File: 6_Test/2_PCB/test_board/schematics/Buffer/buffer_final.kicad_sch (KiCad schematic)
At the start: 15 parts, among them U1 SN74ALVCH162827DLR

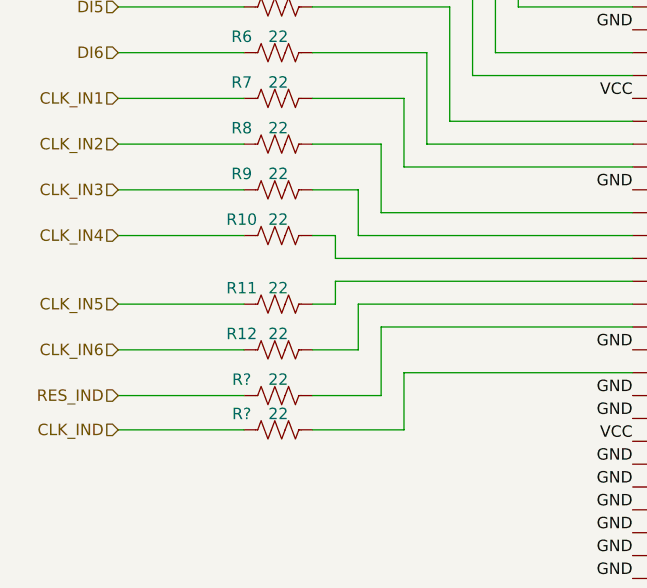
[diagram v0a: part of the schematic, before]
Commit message: Corrections to schematic 11_20_24
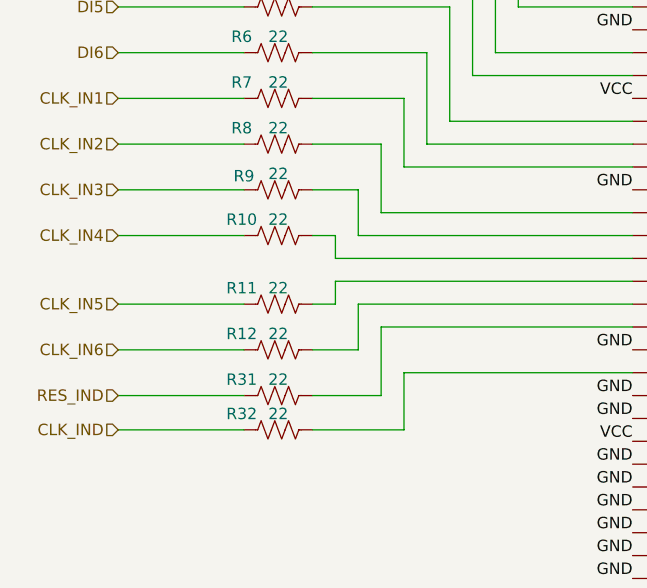
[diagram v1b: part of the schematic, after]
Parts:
- gave numbers to parts that had none: 2
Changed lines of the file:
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@@
 				)
 			)
-			(project "board_main_sim"
-				(path "/9c0580c5-7bd5-4e54-bf4c-826aa4ac3630/49c5ff04-0c5f-41d0-9aa9-a7998c02a6ab"
-					(reference "R10")
+			(project "board_main"
+				(path "/9c0580c5-7bd5-4e54-bf4c-826aa4ac3630/49c5ff04-0c5f-41d0-9aa9-a7998c02a6ab"
+					(reference "R20")
 					(unit 1)
 				)
@@
 				)
 			)
-			(project "board_main_sim"
-				(path "/9c0580c5-7bd5-4e54-bf4c-826aa4ac3630/49c5ff04-0c5f-41d0-9aa9-a7998c02a6ab"
-					(reference "R19")
+			(project "board_main"
+				(path "/9c0580c5-7bd5-4e54-bf4c-826aa4ac3630/49c5ff04-0c5f-41d0-9aa9-a7998c02a6ab"
+					(reference "R29")
 					(unit 1)
 				)
@@
 				)
 			)
-			(project "board_main_sim"
-				(path "/9c0580c5-7bd5-4e54-bf4c-826aa4ac3630/49c5ff04-0c5f-41d0-9aa9-a7998c02a6ab"
-					(reference "R9")
+			(project "board_main"
+				(path "/9c0580c5-7bd5-4e54-bf4c-826aa4ac3630/49c5ff04-0c5f-41d0-9aa9-a7998c02a6ab"
+					(reference "R19")
 					(unit 1)
 				)
@@
 				)
 			)
-			(project "board_main_sim"
-				(path "/9c0580c5-7bd5-4e54-bf4c-826aa4ac3630/49c5ff04-0c5f-41d0-9aa9-a7998c02a6ab"
-					(reference "R12")
+			(project "board_main"
+				(path "/9c0580c5-7bd5-4e54-bf4c-826aa4ac3630/49c5ff04-0c5f-41d0-9aa9-a7998c02a6ab"
+					(reference "R22")
 					(unit 1)
 				)
@@
 				)
 			)
-			(project "board_main_sim"
-				(path "/9c0580c5-7bd5-4e54-bf4c-826aa4ac3630/49c5ff04-0c5f-41d0-9aa9-a7998c02a6ab"
-					(reference "R14")
+			(project "board_main"
+				(path "/9c0580c5-7bd5-4e54-bf4c-826aa4ac3630/49c5ff04-0c5f-41d0-9aa9-a7998c02a6ab"
+					(reference "R24")
 					(unit 1)
 				)
@@
 				)
 			)
-			(project "board_main_sim"
-				(path "/9c0580c5-7bd5-4e54-bf4c-826aa4ac3630/49c5ff04-0c5f-41d0-9aa9-a7998c02a6ab"
-					(reference "R20")
+			(project "board_main"
+				(path "/9c0580c5-7bd5-4e54-bf4c-826aa4ac3630/49c5ff04-0c5f-41d0-9aa9-a7998c02a6ab"
+					(reference "R30")
 					(unit 1)
 				)
@@
 				)
 			)
-			(project "board_main_sim"
-				(path "/9c0580c5-7bd5-4e54-bf4c-826aa4ac3630/49c5ff04-0c5f-41d0-9aa9-a7998c02a6ab"
-					(reference "R13")
+			(project "board_main"
+				(path "/9c0580c5-7bd5-4e54-bf4c-826aa4ac3630/49c5ff04-0c5f-41d0-9aa9-a7998c02a6ab"
+					(reference "R23")
 					(unit 1)
 				)
@@
 		(dnp no)
 		(property "Reference" "R9"
-			(at 84.836 82.042 90)
+			(at 85.09 82.296 90)
 			(effects
 				(font
@@
 				)
 			)
-			(project "board_main_sim"
-				(path "/9c0580c5-7bd5-4e54-bf4c-826aa4ac3630/49c5ff04-0c5f-41d0-9aa9-a7998c02a6ab"
-					(reference "R17")
+			(project "board_main"
+				(path "/9c0580c5-7bd5-4e54-bf4c-826aa4ac3630/49c5ff04-0c5f-41d0-9aa9-a7998c02a6ab"
+					(reference "R27")
 					(unit 1)
 				)
@@
 				)
 			)
-			(project "board_main_sim"
-				(path "/9c0580c5-7bd5-4e54-bf4c-826aa4ac3630/49c5ff04-0c5f-41d0-9aa9-a7998c02a6ab"
-					(reference "R18")
+			(project "board_main"
+				(path "/9c0580c5-7bd5-4e54-bf4c-826aa4ac3630/49c5ff04-0c5f-41d0-9aa9-a7998c02a6ab"
+					(reference "R28")
 					(unit 1)
 				)
@@
 				)
 			)
-			(project "board_main_sim"
-				(path "/9c0580c5-7bd5-4e54-bf4c-826aa4ac3630/49c5ff04-0c5f-41d0-9aa9-a7998c02a6ab"
-					(reference "R15")
+			(project "board_main"
+				(path "/9c0580c5-7bd5-4e54-bf4c-826aa4ac3630/49c5ff04-0c5f-41d0-9aa9-a7998c02a6ab"
+					(reference "R25")
 					(unit 1)
 				)
@@
 				)
 			)
-			(project "board_main_sim"
-				(path "/9c0580c5-7bd5-4e54-bf4c-826aa4ac3630/49c5ff04-0c5f-41d0-9aa9-a7998c02a6ab"
-					(reference "R11")
+			(project "board_main"
+				(path "/9c0580c5-7bd5-4e54-bf4c-826aa4ac3630/49c5ff04-0c5f-41d0-9aa9-a7998c02a6ab"
+					(reference "R21")
 					(unit 1)
 				)
@@
 				)
 			)
-			(project "board_main_sim"
-				(path "/9c0580c5-7bd5-4e54-bf4c-826aa4ac3630/49c5ff04-0c5f-41d0-9aa9-a7998c02a6ab"
-					(reference "U7")
+			(project "board_main"
+				(path "/9c0580c5-7bd5-4e54-bf4c-826aa4ac3630/49c5ff04-0c5f-41d0-9aa9-a7998c02a6ab"
+					(reference "U5")
 					(unit 1)
 				)
@@
 		(on_board yes)
 		(dnp no)
-		(property "Reference" "R?"
+		(property "Reference" "R32"
 			(at 84.836 108.712 90)
 			(effects
@@
 			(project "board_main"
 				(path "/9c0580c5-7bd5-4e54-bf4c-826aa4ac3630/49c5ff04-0c5f-41d0-9aa9-a7998c02a6ab"
-					(reference "R?")
+					(reference "R32")
 					(unit 1)
 				)
@@
 		(on_board yes)
 		(dnp no)
-		(property "Reference" "R?"
+		(property "Reference" "R31"
 			(at 84.836 104.902 90)
 			(effects
@@
 			(project "board_main"
 				(path "/9c0580c5-7bd5-4e54-bf4c-826aa4ac3630/49c5ff04-0c5f-41d0-9aa9-a7998c02a6ab"
-					(reference "R?")
+					(reference "R31")
 					(unit 1)
 				)
@@
 				)
 			)
-			(project "board_main_sim"
-				(path "/9c0580c5-7bd5-4e54-bf4c-826aa4ac3630/49c5ff04-0c5f-41d0-9aa9-a7998c02a6ab"
-					(reference "R16")
-					(unit 1)
-				)
-			)
-		)
-	)
-	(sheet_instances
-		(path "/"
-			(page "1")
-		)
-	)
+			(project "board_main"
+				(path "/9c0580c5-7bd5-4e54-bf4c-826aa4ac3630/49c5ff04-0c5f-41d0-9aa9-a7998c02a6ab"
+					(reference "R26")
+					(unit 1)
+				)
+			)
+		)
+	)
